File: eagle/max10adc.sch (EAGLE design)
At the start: 203 parts, among them IC1 MAX19506, IC2 MAX19506, J1 MOLEX_BNC_73100-0105, J2 MOLEX_BNC_73100-0105, J3 MOLEX_BNC_73100-0105, J4 MOLEX_BNC_73100-0105, K1 AQY21SOP, K2 AQY21SOP, K3 AQY21SOP, K4 AQY21SOP, K5 AQY21SOP, K6 AQY21SOP, K7 AQY21SOP, K8 AQY21SOP, U1 MAX4416ESA, U2 MAX4416ESA, U340G CH340G, Y1 ABL-12.000MHZ-B2

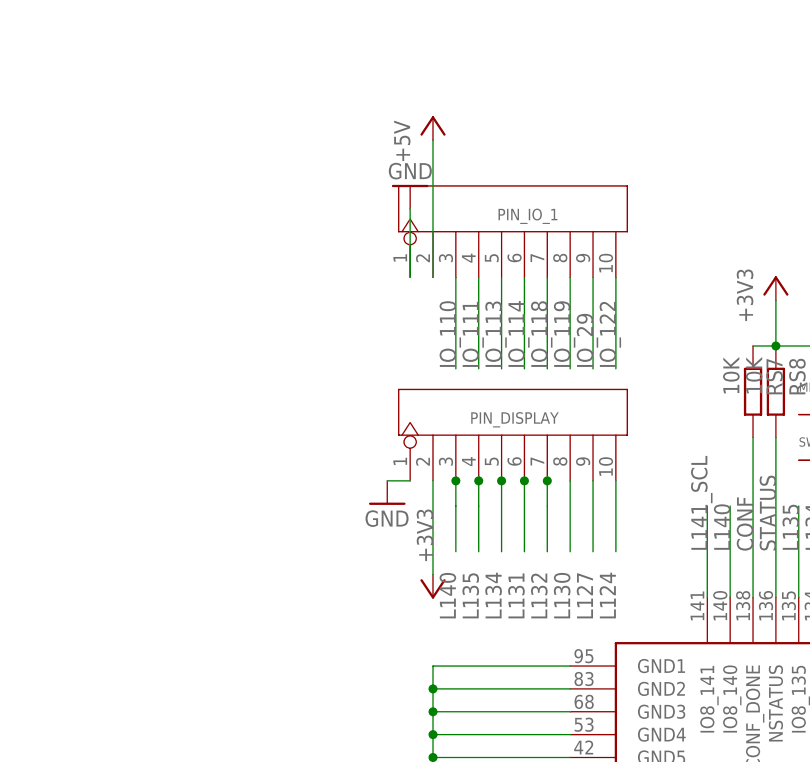
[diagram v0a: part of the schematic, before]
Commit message: for 8.7 and USB2
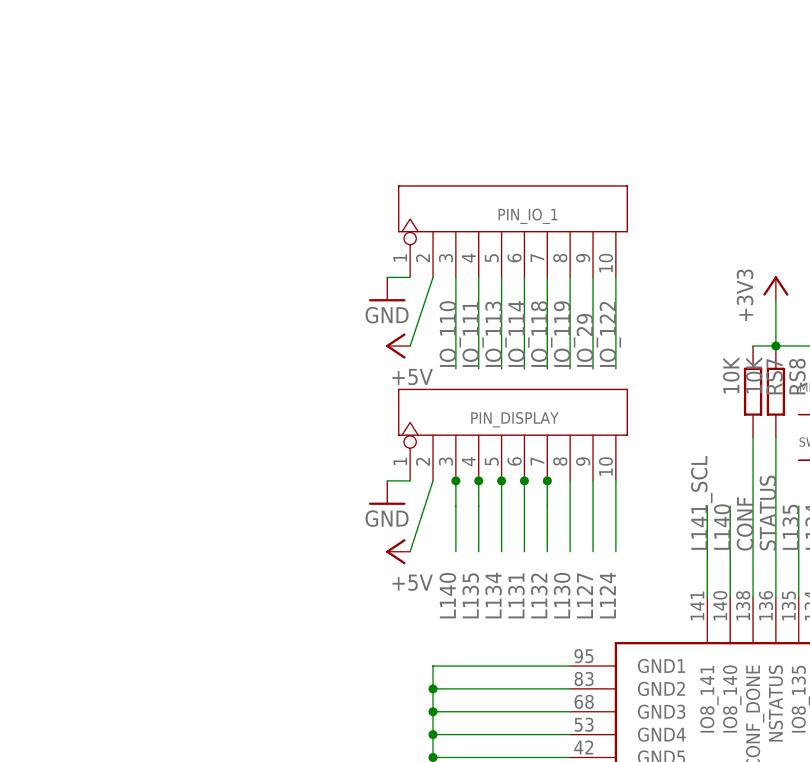
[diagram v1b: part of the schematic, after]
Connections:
- net +3V3: no longer PIN_DISPLAY.2
- net +5V: now also PIN_DISPLAY.2
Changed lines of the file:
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@@
 <part name="USB1" library="PP_Connectors" deviceset="USB_5PIN" device="_10118193-0001LF" value="MF-CON-MICROUSB-RIGHT"/>
 <part name="GND42" library="supply1" deviceset="GND" device=""/>
-<part name="+3V22" library="supply1" deviceset="+3V3" device=""/>
 <part name="SW_RESET" library="MF_Switches" deviceset="TACT" device="_4.2MM" value="MF-SW-TACT-4.2MM"/>
 <part name="+3V16" library="supply1" deviceset="+3V3" device=""/>
@@
 <attribute name="MPN" value="MF-CAP-0805-1uF"/>
 </part>
+<part name="P+6" library="supply1" deviceset="+5V" device=""/>
 </parts>
 <sheets>
@@
 <instance part="USB1" gate="G$1" x="-375.92" y="-104.14"/>
 <instance part="GND42" gate="1" x="-480.06" y="78.994"/>
-<instance part="+3V22" gate="G$1" x="-474.98" y="68.58" smashed="yes" rot="R180">
-<attribute name="VALUE" x="-474.98" y="72.39" size="1.778" layer="96" rot="R90"/>
-</instance>
 <instance part="SW_RESET" gate="G$1" x="-431.8" y="86.36" smashed="yes">
 <attribute name="NAME" x="-434.34" y="86.36" size="1.016" layer="95" font="vector" align="top-left"/>
@@
 <attribute name="NAME" x="-461.01" y="111.76" size="1.27" layer="95" ratio="10" rot="R180"/>
 </instance>
-<instance part="P+7" gate="1" x="-474.98" y="121.92"/>
-<instance part="GND68" gate="1" x="-477.52" y="114.3" rot="R180"/>
+<instance part="P+7" gate="1" x="-480.06" y="96.52" rot="R90"/>
+<instance part="GND68" gate="1" x="-480.06" y="101.6"/>
 <instance part="GND69" gate="1" x="-355.6" y="-116.84" rot="R90"/>
 <instance part="K1" gate="G$1" x="-228.6" y="-104.14" rot="R180"/>
@@
 <attribute name="MPN" x="-596.9" y="-60.96" size="1.778" layer="96" display="off"/>
 </instance>
+<instance part="P+6" gate="1" x="-480.06" y="73.66" rot="R90"/>
 </instances>
 <busses>
@@
 <pinref part="PIN_IO_1" gate="G$1" pin="2"/>
 <pinref part="P+7" gate="1" pin="+5V"/>
-<wire x1="-474.98" y1="119.38" x2="-474.98" y2="104.14" width="0.1524" layer="91"/>
+<wire x1="-477.52" y1="96.52" x2="-474.98" y2="104.14" width="0.1524" layer="91"/>
 </segment>
 <segment>
@@
 <pinref part="P+4" gate="1" pin="+5V"/>
 <wire x1="-337.82" y1="-127" x2="-337.82" y2="-121.92" width="0.1524" layer="91"/>
+</segment>
+<segment>
+<pinref part="PIN_DISPLAY" gate="G$1" pin="2"/>
+<wire x1="-477.52" y1="73.66" x2="-474.98" y2="81.534" width="0.1524" layer="91"/>
+<pinref part="P+6" gate="1" pin="+5V"/>
 </segment>
 </net>
@@
 <pinref part="PIN_IO_1" gate="G$1" pin="1"/>
 <pinref part="GND68" gate="1" pin="GND"/>
-<wire x1="-477.52" y1="111.76" x2="-477.52" y2="104.14" width="0.1524" layer="91"/>
+<wire x1="-480.06" y1="104.14" x2="-477.52" y2="104.14" width="0.1524" layer="91"/>
 </segment>
 <segment>
@@
 <junction x="-393.7" y="-142.24"/>
 </segment>
-<segment>
-<pinref part="+3V22" gate="G$1" pin="+3V3"/>
-<pinref part="PIN_DISPLAY" gate="G$1" pin="2"/>
-<wire x1="-474.98" y1="71.12" x2="-474.98" y2="81.534" width="0.1524" layer="91"/>
-</segment>
 </net>
